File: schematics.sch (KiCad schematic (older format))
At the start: 18 parts, among them P1 Host_in, P2 UI, P3 Host_out, U1 MIDI_Dec, U10 ADSR, U11 Gate, U12 Mult, U13 ADSR, U14 Mult, U15 Mix, U2 LFO, U3 ADSR, U4 Mult, U5 Mult, U6 Mult, U7 Wavesource, U8 Add, U9 Filter

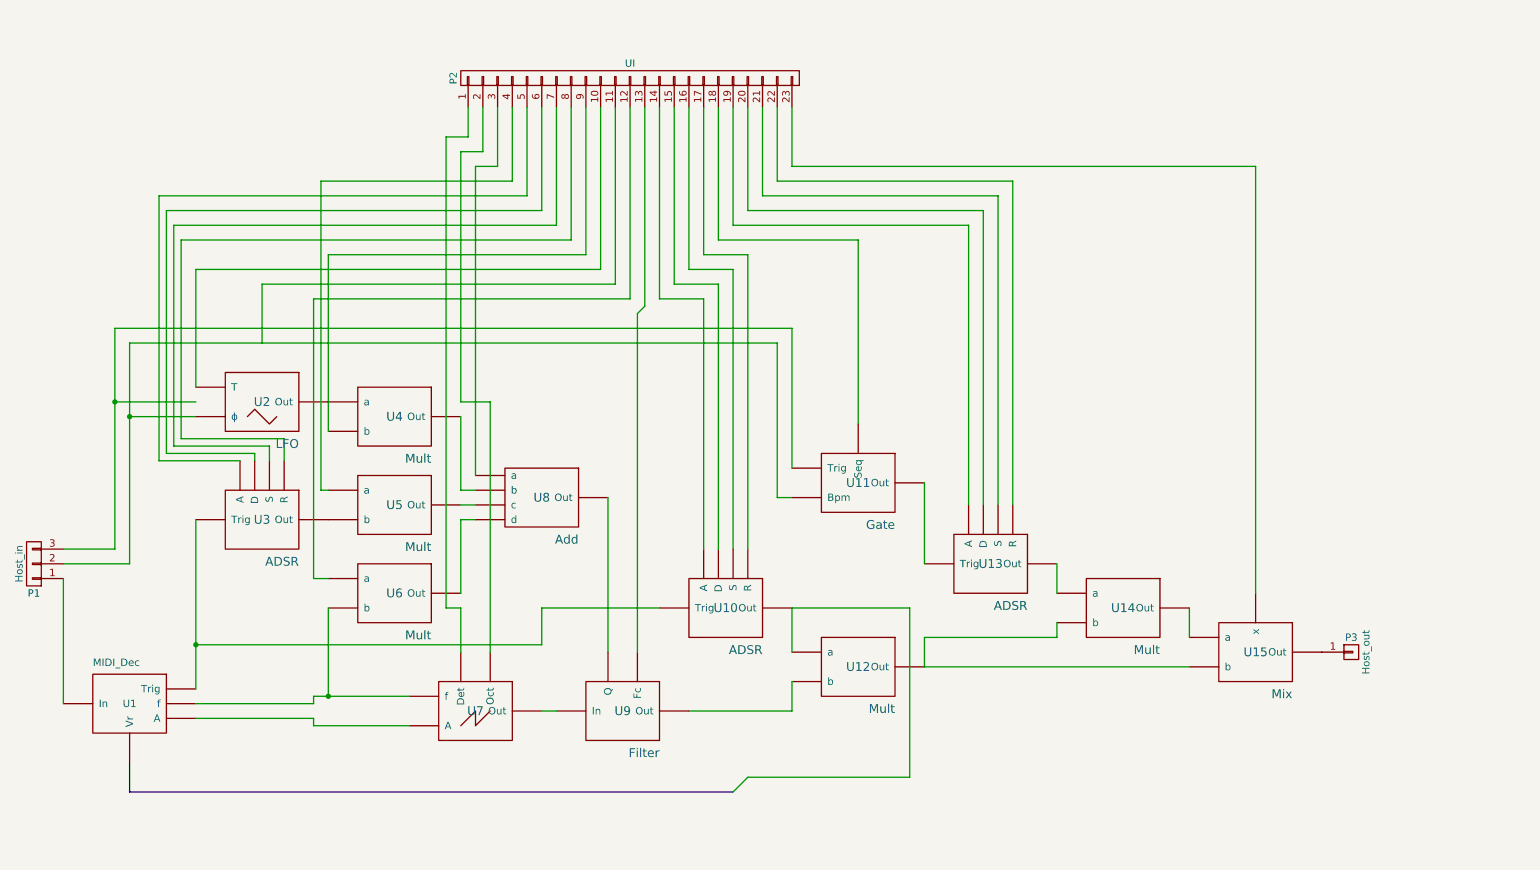
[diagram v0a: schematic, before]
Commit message: New schematics for 'voice card' only
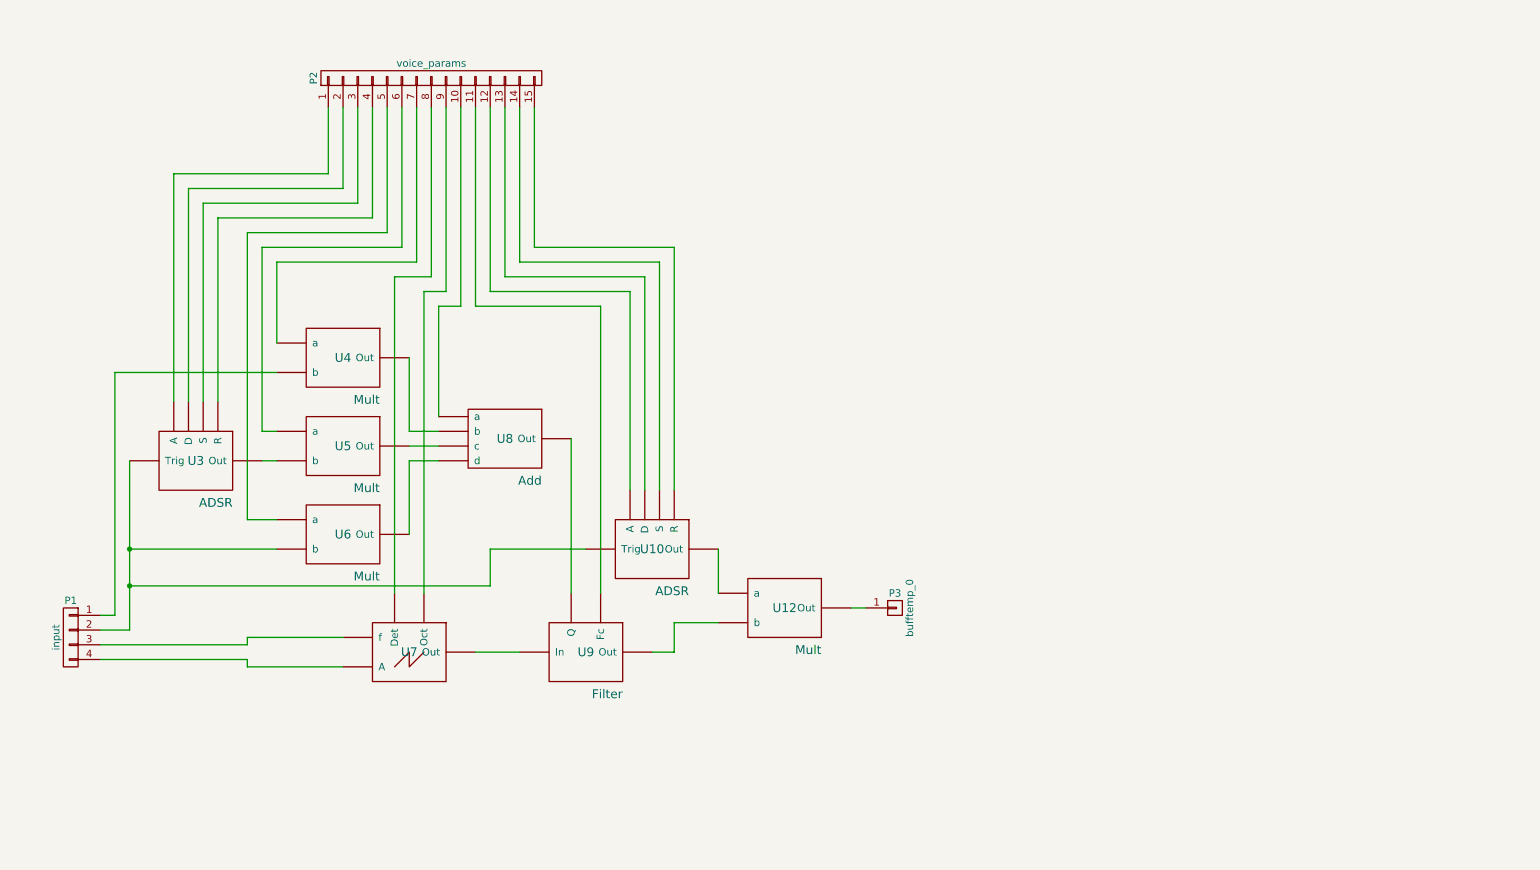
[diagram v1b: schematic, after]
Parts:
- removed P1: Host_in, symbol CONN_01X03
- removed P2: UI, symbol CONN_01X23
- removed U1: MIDI_Dec, symbol MIDI_Dec
- removed U11: Gate, symbol Gate
- removed U13: ADSR, symbol ADSR
- removed U14: Mult, symbol Mult
- removed U15: Mix, symbol Mix
- removed U2: LFO, symbol LFO
- added P1: input, symbol CONN_01X04
- added P2: voice_params, symbol CONN_01X15
- P3: value Host_out -> bufftemp_0
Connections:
- net at U7.~ (Out): now also P2.9 (P9)
- net at U6.~ (Out): now also P2.5 (P5); no longer U7.~ (Out)
- net at U9.~ (Q): now also P2.11 (P11); no longer U7.~ (Out)
- net at U3.~ (Trig): now also P2.4 (P4); no longer U10.~ (Trig)
- net at U12.~ (Out): now also P3.1 (P1)
- net at U10.~ (Trig): now also P2.15 (P15); no longer U12.~ (Out)
- net at U5.~ (Out): now also P2.6 (P6); no longer U3.~ (Trig)
- net at U8.~ (Out): now also P2.10 (P10); no longer U5.~ (Out)
- net at U4.~ (Out): now also P2.7 (P7)
- new net: U7.~ (Out), U9.~ (Q)
- new net: P1.3 (P3), U7.~ (Out)
- new net: P1.4 (P4), U7.~ (Out)
- new net: P2.8 (P8), U7.~ (Out)
- new net: U10.~ (Trig), U12.~ (Out)
- new net: U12.~ (Out), U9.~ (Q)
- new net: U3.~ (Trig), U5.~ (Out)
- new net: U5.~ (Out), U8.~ (Out)
- new net: P1.2 (P2), U10.~ (Trig), U3.~ (Trig), U6.~ (Out)
- new net: U6.~ (Out), U8.~ (Out)
- new net: P2.1 (P1), U3.~ (Trig)
- new net: P2.2 (P2), U3.~ (Trig)
- new net: P2.3 (P3), U3.~ (Trig)
- new net: P2.12 (P12), U10.~ (Trig)
- new net: P2.13 (P13), U10.~ (Trig)
- new net: P2.14 (P14), U10.~ (Trig)
- new net: U8.~ (Out), U9.~ (Q)
- new net: U4.~ (Out), U8.~ (Out)
- new net: P1.1 (P1), U4.~ (Out)
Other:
- moved on the sheet: U10, U12, U3, U4, U5, U6, U7, U8, U9

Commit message: New schematics
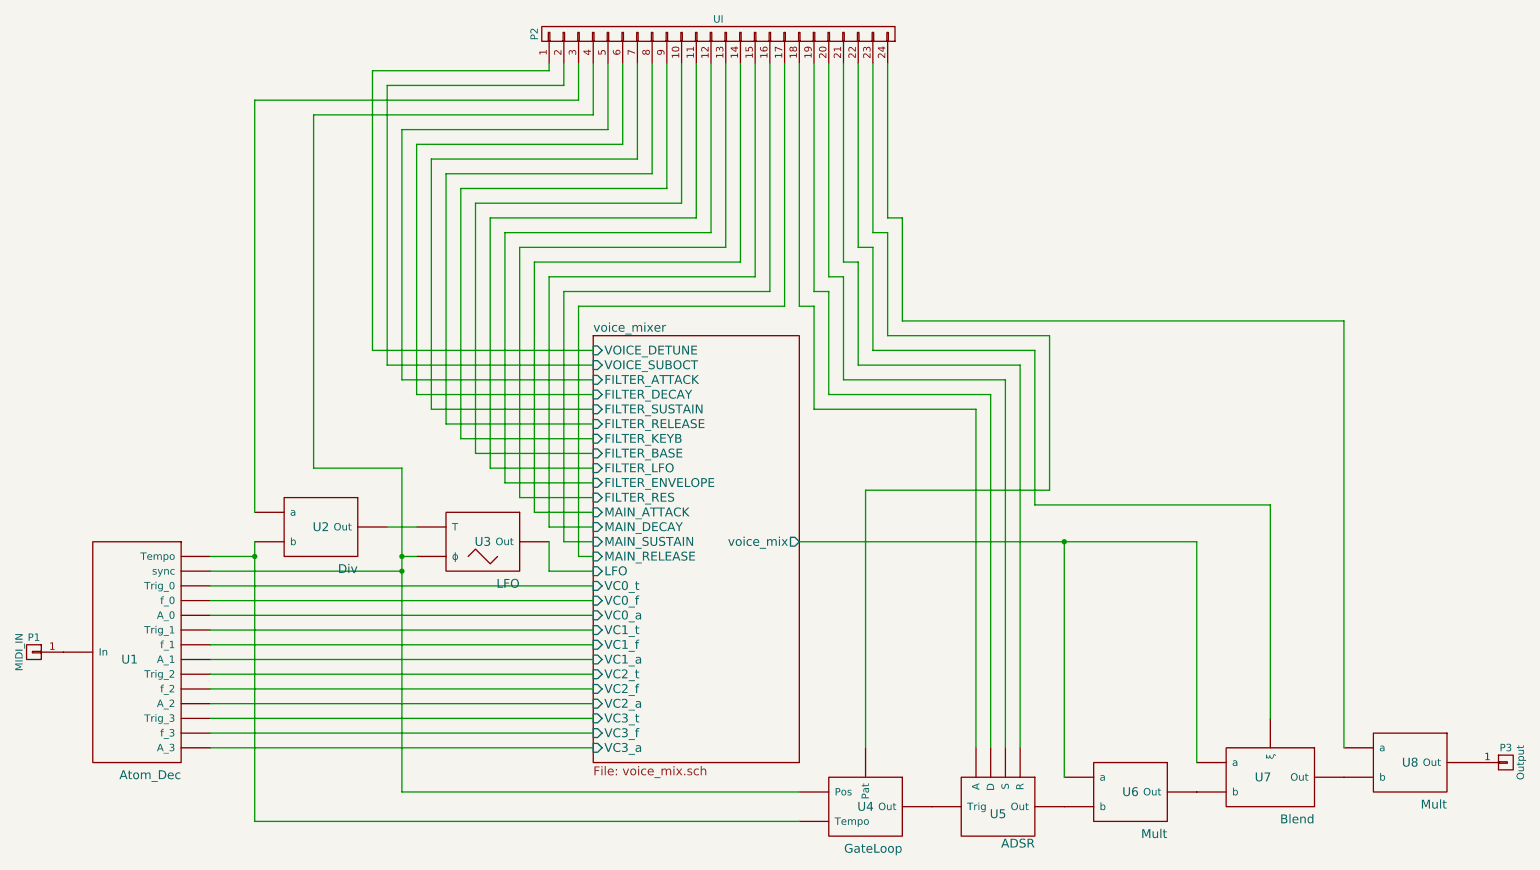
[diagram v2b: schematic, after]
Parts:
- removed P1: input, symbol CONN_01X04
- removed P2: voice_params, symbol CONN_01X15
- removed U10, U3: ADSR, symbol ADSR
- removed U12, U4, U5: Mult, symbol Mult
- removed U7: Wavesource, symbol Wavesource
- removed U8: Add, symbol Add
- removed U9: Filter, symbol Filter
- added P1: MIDI_IN, symbol CONN_01X01
- added P2: UI, symbol CONN_01X24
- added U1: Atom_Dec, symbol Atom_Dec
- added U2: Div, symbol Div
- added U3: LFO, symbol LFO
- added U4: GateLoop, symbol GateLoop
- added U5: ADSR, symbol ADSR
- added U7: Blend, symbol Blend
- added U8: Mult, symbol Mult
- P3: value bufftemp_0 -> Output
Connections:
- net at P3.1 (P1): now also U8.~ (Out)
- net voice_mixer/voice_mix: now reaches U6.~ (Out)
- net voice_mixer/voice_mix: now also U7.~ (ξ)
- new net: U5.~ (Trig), U6.~ (Out)
- new net: U6.~ (Out), U7.~ (ξ)
- new net: P2.4 (P4), U1.~ (Trig_3), U3.~ (ϕ), U4.~ (Tempo)
- new net: U2.~ (Out), U3.~ (ϕ)
- new net: U1.~ (Trig_3), U2.~ (Out), U4.~ (Tempo)
- new net: P1.1 (P1), U1.~ (Trig_3)
- new net: U4.~ (Tempo), U5.~ (Trig)
- new net: P2.18 (P18), U5.~ (Trig)
- new net: P2.19 (P19), U5.~ (Trig)
- new net: P2.20 (P20), U5.~ (Trig)
- new net: P2.21 (P21), U5.~ (Trig)
- new net: P2.3 (P3), U2.~ (Out)
- new net: P2.23 (P23), U4.~ (Tempo)
- new net: U7.~ (ξ), U8.~ (Out)
- new net: P2.22 (P22), U7.~ (ξ)
- new net: P2.24 (P24), U8.~ (Out)
- new net voice_mixer/FILTER_ATTACK: P2.5 (P5)
- new net voice_mixer/FILTER_BASE: P2.10 (P10)
- new net voice_mixer/FILTER_DECAY: P2.6 (P6)
- new net voice_mixer/FILTER_ENVELOPE: P2.12 (P12)
- new net voice_mixer/FILTER_KEYB: P2.9 (P9)
- new net voice_mixer/FILTER_LFO: P2.11 (P11)
- new net voice_mixer/FILTER_RELEASE: P2.8 (P8)
- new net voice_mixer/FILTER_RES: P2.13 (P13)
- new net voice_mixer/FILTER_SUSTAIN: P2.7 (P7)
- new net voice_mixer/LFO: U3.~ (ϕ)
- new net voice_mixer/MAIN_ATTACK: P2.14 (P14)
- new net voice_mixer/MAIN_DECAY: P2.15 (P15)
- new net voice_mixer/MAIN_RELEASE: P2.17 (P17)
- new net voice_mixer/MAIN_SUSTAIN: P2.16 (P16)
- new net voice_mixer/VC0_a: U1.~ (Trig_3)
- new net voice_mixer/VC0_f: U1.~ (Trig_3)
- new net voice_mixer/VC0_t: U1.~ (Trig_3)
- new net voice_mixer/VC1_a: U1.~ (Trig_3)
- new net voice_mixer/VC1_f: U1.~ (Trig_3)
- new net voice_mixer/VC1_t: U1.~ (Trig_3)
- new net voice_mixer/VC2_a: U1.~ (Trig_3)
- new net voice_mixer/VC2_f: U1.~ (Trig_3)
- new net voice_mixer/VC2_t: U1.~ (Trig_3)
- new net voice_mixer/VC3_a: U1.~ (Trig_3)
- new net voice_mixer/VC3_f: U1.~ (Trig_3)
- new net voice_mixer/VC3_t: U1.~ (Trig_3)
- new net voice_mixer/VOICE_DETUNE: P2.1 (P1)
- new net voice_mixer/VOICE_SUBOCT: P2.2 (P2)
